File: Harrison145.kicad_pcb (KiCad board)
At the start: 2 copper layers, 85 x 55 mm, 152 parts, among them J1 PITCH ANTENNA, J2 VOLUME ANTENNA, J3 GROUND POINT, J4 LINE OUT, J5 9V IN, Q1 MMBT3906, Q10 SMP5484, Q11 MMBT3906, Q12 MMBT3906, Q13 SMP5484, Q14 MMBT3904, Q15 MMBT3904, Q16 MMBT3906, Q2 MMBT3906, Q3 SMP5484, Q4 MMBT3904, Q5 SMP5484, Q6 MMBT3906, Q7 MMBT3906, Q8 SMP5484, Q9 MMBT3904, U1 LDK320-ADJ_SOT23_SOT353

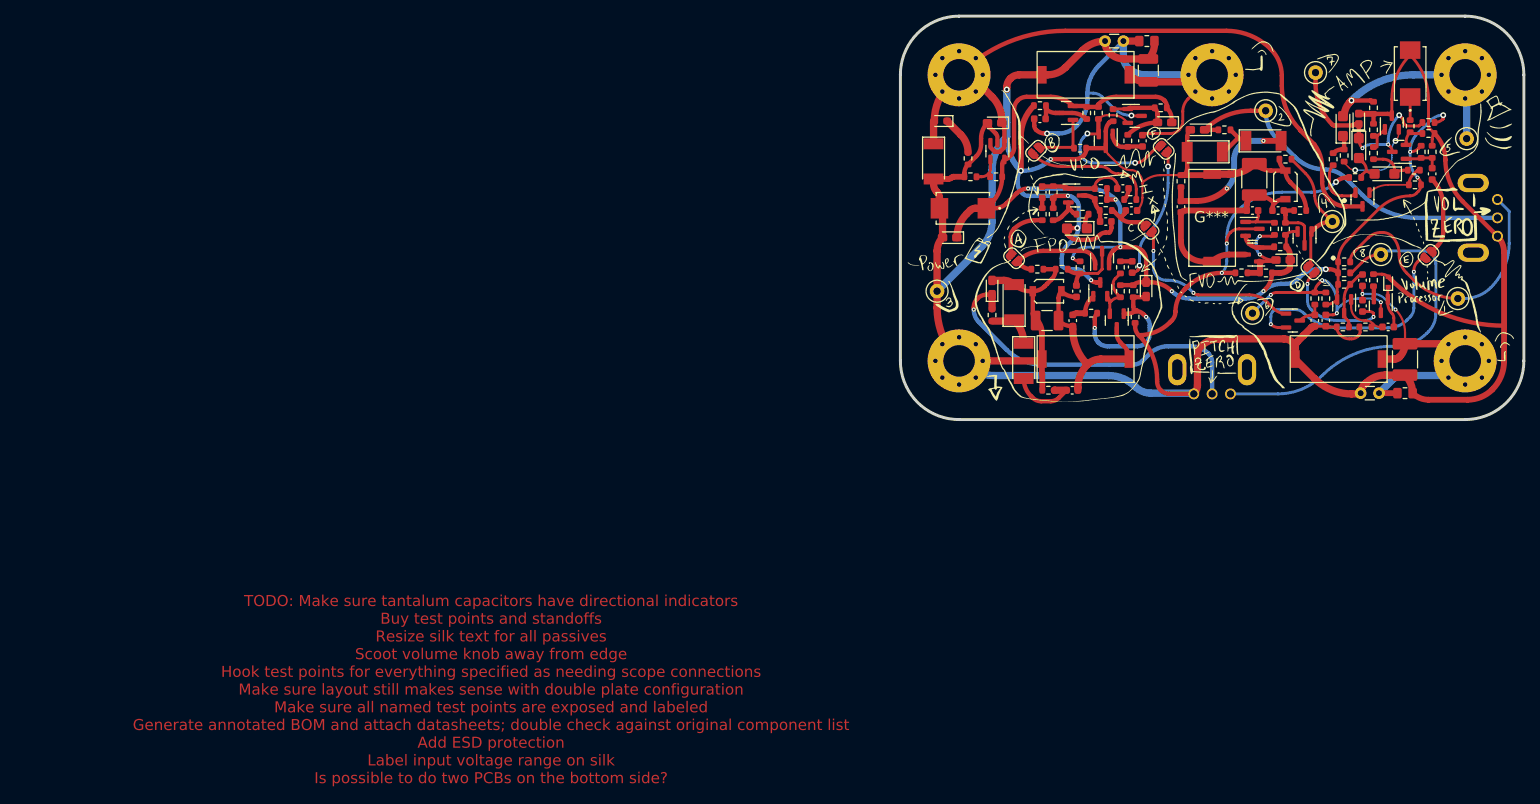
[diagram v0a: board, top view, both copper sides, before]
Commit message: All DRC/ERC that matters passes
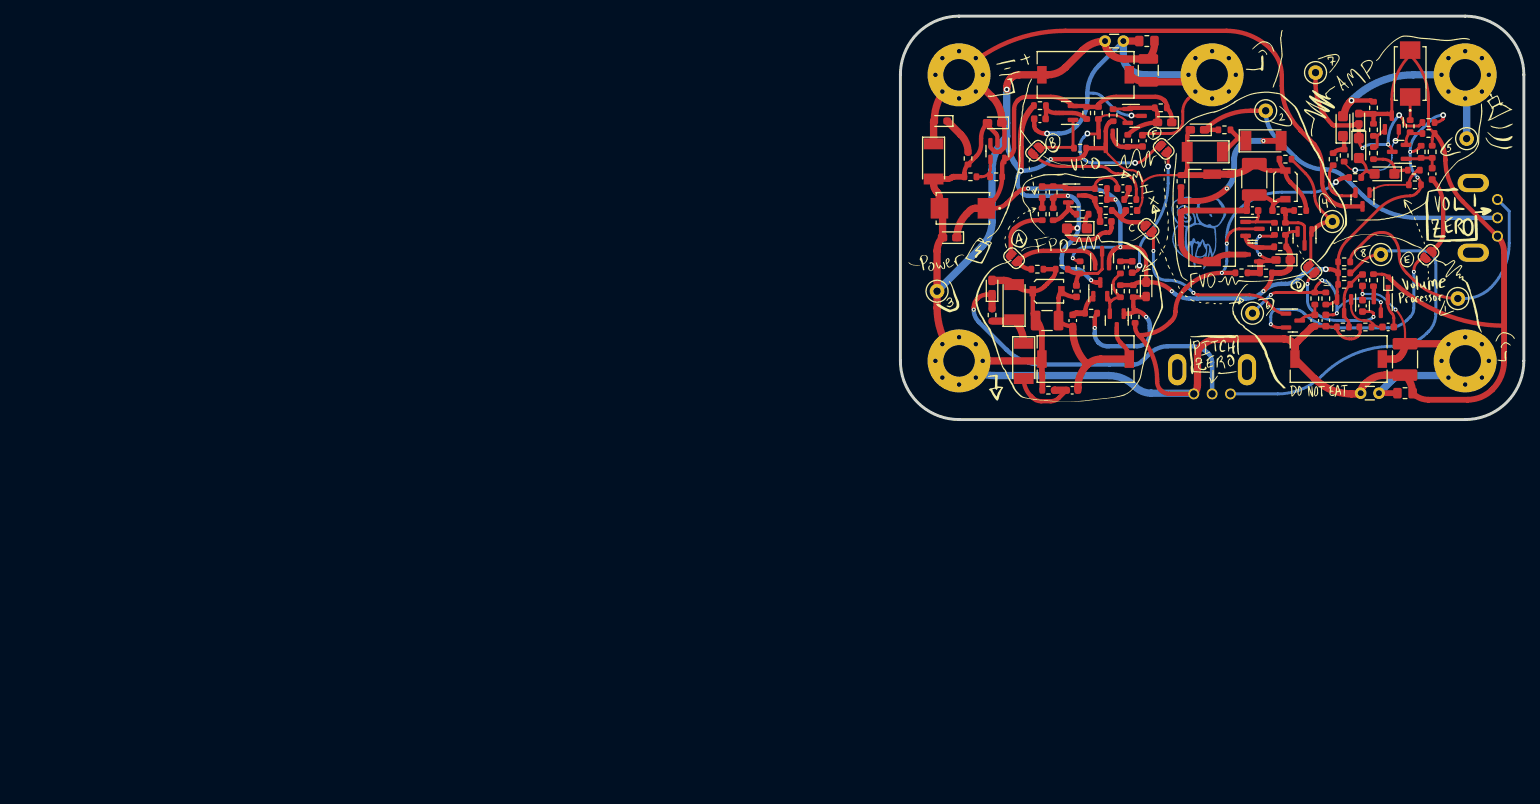
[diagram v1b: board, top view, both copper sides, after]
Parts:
- added G***: LOGO, Theremin:walrus, B.Cu at (160.5, 50.1)
- moved Ge 0.10 mm to (183.0, 79.4)
- turned R43 to 0 degrees
- renumbered G*** to Ge
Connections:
- R43 pad 1: +7.5V -> Net-(C36-Pad1)
- R43 pad 2: Net-(C36-Pad1) -> +7.5V
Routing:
- net Net-(C37-Pad2): track 5.33 -> 4.50 mm
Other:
- board text removed: "AMP"
- board text removed: "FPO"
- board text removed: "TODO: Make sure tantalum capacitors have directional indicators Buy test points and standoffs Resize silk text for all passives Scoot volume knob away from edge Hook test points for everything specified as needing scope connections Make sure layout still makes sense with double plate configuration Make sure all named test points are exposed and labeled Generate annotated BOM and attach datasheets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"
- board text removed: "VPO"
- board text removed: "VVO"
